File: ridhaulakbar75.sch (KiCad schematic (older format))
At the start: 204 parts, among them J1 Conn_01x04, J2 AVR-ISP-6, U1 TEENSY2.0

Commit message: big update
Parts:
- removed C1, C10, C11, C12, C13, C14, C15, C16, C17, C18, C2, C3, C4, C5, C6, C7, C8, C9: 0.1uF, Capacitor_SMD:C_0603_1608Metric_Pad1.05x0.95mm_HandSolder, symbol Device:C_Small
- removed D71: 1N4148W, master-Keebio-Parts:D_SOD-123-v2, symbol Diode:1N4148W
- removed J2: AVR-ISP-6, random-keyboard-parts:Reset_Pretty-Mask, symbol Connector:AVR-ISP-6
- removed LED1, LED10, LED11, LED12, LED13, LED14, LED15, LED16, LED17, LED18, LED2, LED3, LED4, LED5, LED6, LED7, LED8, LED9: WS2812B, WS2812B:WS2812B, symbol ws2812b:WS2812B
- removed MX71: Prnt Scr, MX_Only:MXOnly-1U-NoLED, symbol MX_Alps_Hybrid:MX-NoLED
- removed U1: TEENSY2.0, master-Keebio-Parts:Teensy_2.0, symbol keyboard_parts:TEENSY2.0
- added D82: BLUE, LED_SMD:LED_0603_1608Metric, symbol Device:LED
- added D83: 1N5819, Diode_SMD:D_SOD-323F, symbol Device:D_Schottky_Small
- added D84: RED, LED_SMD:LED_0603_1608Metric, symbol Device:LED
- added F1: 500mA, Fuse:Fuse_1206_3216Metric, symbol Device:Polyfuse_Small
- added J2: Ex_Bat, Connector_PinHeader_2.54mm:PinHeader_1x02_P2.54mm_Vertical, symbol Connector_Generic:Conn_01x02
- added J3: Ex_USB, nrfmicro:connector_usb, symbol Connector_Generic:Conn_01x04
- added Q1, Q2: AO3407, Package_TO_SOT_SMD:SOT-23, symbol Device:Q_PMOS_GSD
- added R1, R2: 5.1k, Resistor_SMD:R_0603_1608Metric, symbol Device:R_Small
- added R3: 820K, Resistor_SMD:R_0603_1608Metric, symbol Device:R_Small
- added R4, R8: 1K, Resistor_SMD:R_0603_1608Metric, symbol Device:R_Small
- added R5, R6: 2M, Resistor_SMD:R_0603_1608Metric, symbol Device:R_Small
- added R7: 100k, Resistor_SMD:R_0603_1608Metric, symbol Device:R_Small
- added R9: 2K, Resistor_SMD:R_0603_1608Metric, symbol Device:R_Small
- added SW1: Rotary_Encoder_Switch, master-Keebio-Parts:RotaryEncoder_EC11-no-legs, symbol Device:Rotary_Encoder_Switch
- added U1: USBLC6-2SC6, Package_TO_SOT_SMD:SOT-23-6, symbol Power_Protection:USBLC6-2SC6
- added U2: E73-2G4M08S1C-52840, nrfmicro:E73-2G4M08S1C-52840, symbol nrfmicro:E73-2G4M08S1C-52840
- added U3: XC6220B331MR, Package_TO_SOT_SMD:SOT-23-5, symbol Regulator_Linear:XC6220B331MR
- added U4: TP4054, Package_TO_SOT_SMD:SOT-23-5, symbol Battery_Management:MCP73831-3-OT
- added Y1: 32.768kHz, Crystal:Crystal_SMD_MicroCrystal_CM9V-T1A-2Pin_1.6x1.0mm, symbol Device:Crystal_Small
- J1: value Conn_01x04 -> SWD; footprint Connector_PinHeader_2.54mm:PinHeader_1x04_P2.54mm_Vertical -> nrfmicro:connector_swd
- MX1, MX18: footprint MX_Only:MXOnly-1U-NoLED -> MX_Only:MXOnly-1U-Hotswap
- MX10: renamed from MX49; footprint MX_Only:MXOnly-1U-NoLED -> MX_Only:MXOnly-1U-Hotswap
- MX11: renamed from MX54; footprint MX_Only:MXOnly-1U-NoLED -> MX_Only:MXOnly-1U-Hotswap
- MX12: renamed from MX60; footprint MX_Only:MXOnly-1U-NoLED -> MX_Only:MXOnly-1U-Hotswap
- MX13: renamed from MX66; footprint MX_Only:MXOnly-1U-NoLED -> MX_Only:MXOnly-1U-Hotswap
- MX14: renamed from MX77; footprint MX_Only:MXOnly-1U-NoLED -> MX_Only:MXOnly-1U-Hotswap
- MX15: renamed from MX2; footprint MX_Only:MXOnly-1U-NoLED -> MX_Only:MXOnly-1U-Hotswap
- MX16: renamed from MX8; footprint MX_Only:MXOnly-1U-NoLED -> MX_Only:MXOnly-1U-Hotswap
- MX17: renamed from MX13; footprint MX_Only:MXOnly-1U-NoLED -> MX_Only:MXOnly-1U-Hotswap
- MX19: renamed from MX24; footprint MX_Only:MXOnly-1U-NoLED -> MX_Only:MXOnly-1U-Hotswap
- MX2: renamed from MX7; footprint MX_Only:MXOnly-1U-NoLED -> MX_Only:MXOnly-1U-Hotswap
- MX20: renamed from MX29; footprint MX_Only:MXOnly-1U-NoLED -> MX_Only:MXOnly-1U-Hotswap
- MX21: renamed from MX34; footprint MX_Only:MXOnly-1U-NoLED -> MX_Only:MXOnly-1U-Hotswap
- MX22: renamed from MX40; footprint MX_Only:MXOnly-1U-NoLED -> MX_Only:MXOnly-1U-Hotswap
- MX23: renamed from MX45; footprint MX_Only:MXOnly-1U-NoLED -> MX_Only:MXOnly-1U-Hotswap
- MX24: renamed from MX50; footprint MX_Only:MXOnly-1U-NoLED -> MX_Only:MXOnly-1U-Hotswap
- MX25: renamed from MX55; footprint MX_Only:MXOnly-1U-NoLED -> MX_Only:MXOnly-1U-Hotswap
- MX26: renamed from MX61; footprint MX_Only:MXOnly-1U-NoLED -> MX_Only:MXOnly-1U-Hotswap
- MX27: renamed from MX67; footprint MX_Only:MXOnly-1U-NoLED -> MX_Only:MXOnly-1U-Hotswap
- MX28: renamed from MX72; footprint MX_Only:MXOnly-2U-NoLED -> MX_Only:MXOnly-2U-Hotswap
- MX29: renamed from MX78; footprint MX_Only:MXOnly-1U-NoLED -> MX_Only:MXOnly-1U-Hotswap
- MX3: renamed from MX12; footprint MX_Only:MXOnly-1U-NoLED -> MX_Only:MXOnly-1U-Hotswap
- MX30: renamed from MX3; footprint MX_Only:MXOnly-1.5U-NoLED -> MX_Only:MXOnly-1.5U-Hotswap
- MX31: renamed from MX9; footprint MX_Only:MXOnly-1U-NoLED -> MX_Only:MXOnly-1U-Hotswap
- MX32: renamed from MX14; footprint MX_Only:MXOnly-1U-NoLED -> MX_Only:MXOnly-1U-Hotswap
- MX33: renamed from MX19; footprint MX_Only:MXOnly-1U-NoLED -> MX_Only:MXOnly-1U-Hotswap
- MX34: renamed from MX25; footprint MX_Only:MXOnly-1U-NoLED -> MX_Only:MXOnly-1U-Hotswap
- MX35: renamed from MX30; footprint MX_Only:MXOnly-1U-NoLED -> MX_Only:MXOnly-1U-Hotswap
- MX36: renamed from MX35; footprint MX_Only:MXOnly-1U-NoLED -> MX_Only:MXOnly-1U-Hotswap
- MX37: renamed from MX41; footprint MX_Only:MXOnly-1U-NoLED -> MX_Only:MXOnly-1U-Hotswap
- MX38: renamed from MX46; footprint MX_Only:MXOnly-1U-NoLED -> MX_Only:MXOnly-1U-Hotswap
- MX39: renamed from MX51; footprint MX_Only:MXOnly-1U-NoLED -> MX_Only:MXOnly-1U-Hotswap
- MX4: renamed from MX17; footprint MX_Only:MXOnly-1U-NoLED -> MX_Only:MXOnly-1U-Hotswap
- MX40: renamed from MX56; footprint MX_Only:MXOnly-1U-NoLED -> MX_Only:MXOnly-1U-Hotswap
- MX41: renamed from MX62; footprint MX_Only:MXOnly-1U-NoLED -> MX_Only:MXOnly-1U-Hotswap
- MX42: renamed from MX68; footprint MX_Only:MXOnly-1U-NoLED -> MX_Only:MXOnly-1U-Hotswap
- MX43: renamed from MX73; footprint MX_Only:MXOnly-1.5U-NoLED -> MX_Only:MXOnly-1.5U-Hotswap
- MX44: renamed from MX79; footprint MX_Only:MXOnly-1U-NoLED -> MX_Only:MXOnly-1U-Hotswap
- MX45: renamed from MX4; footprint MX_Only:MXOnly-1.75U-NoLED -> MX_Only:MXOnly-1.75U-Hotswap
- MX46: renamed from MX10; footprint MX_Only:MXOnly-1U-NoLED -> MX_Only:MXOnly-1U-Hotswap
- MX47: renamed from MX15; footprint MX_Only:MXOnly-1U-NoLED -> MX_Only:MXOnly-1U-Hotswap
- MX48: renamed from MX20; footprint MX_Only:MXOnly-1U-NoLED -> MX_Only:MXOnly-1U-Hotswap
- MX49: renamed from MX26; footprint MX_Only:MXOnly-1U-NoLED -> MX_Only:MXOnly-1U-Hotswap
- MX5: renamed from MX23; footprint MX_Only:MXOnly-1U-NoLED -> MX_Only:MXOnly-1U-Hotswap
- MX50: renamed from MX31; footprint MX_Only:MXOnly-1U-NoLED -> MX_Only:MXOnly-1U-Hotswap
- MX51: renamed from MX36; footprint MX_Only:MXOnly-1U-NoLED -> MX_Only:MXOnly-1U-Hotswap
- MX52: renamed from MX42; footprint MX_Only:MXOnly-1U-NoLED -> MX_Only:MXOnly-1U-Hotswap
- MX53: renamed from MX47; footprint MX_Only:MXOnly-1U-NoLED -> MX_Only:MXOnly-1U-Hotswap
- MX54: renamed from MX52; footprint MX_Only:MXOnly-1U-NoLED -> MX_Only:MXOnly-1U-Hotswap
- MX55: renamed from MX57; footprint MX_Only:MXOnly-1U-NoLED -> MX_Only:MXOnly-1U-Hotswap
- MX56: renamed from MX63; footprint MX_Only:MXOnly-1U-NoLED -> MX_Only:MXOnly-1U-Hotswap
- MX57: renamed from MX74; footprint MX_Only:MXOnly-2.25U-NoLED -> MX_Only:MXOnly-2.25U-Hotswap
- MX58: renamed from MX80; footprint MX_Only:MXOnly-1U-NoLED -> MX_Only:MXOnly-1U-Hotswap
- MX59: renamed from MX5; footprint MX_Only:MXOnly-2.25U-NoLED -> MX_Only:MXOnly-2.25U-Hotswap
- MX6: renamed from MX28; footprint MX_Only:MXOnly-1U-NoLED -> MX_Only:MXOnly-1U-Hotswap
- MX60: renamed from MX16; footprint MX_Only:MXOnly-1U-NoLED -> MX_Only:MXOnly-1U-Hotswap
- MX61: renamed from MX21; footprint MX_Only:MXOnly-1U-NoLED -> MX_Only:MXOnly-1U-Hotswap
- MX62: renamed from MX27; footprint MX_Only:MXOnly-1U-NoLED -> MX_Only:MXOnly-1U-Hotswap
- MX63: renamed from MX32; footprint MX_Only:MXOnly-1U-NoLED -> MX_Only:MXOnly-1U-Hotswap
- MX64: renamed from MX37; footprint MX_Only:MXOnly-1U-NoLED -> MX_Only:MXOnly-1U-Hotswap
- MX65: renamed from MX43; footprint MX_Only:MXOnly-1U-NoLED -> MX_Only:MXOnly-1U-Hotswap
- MX66: renamed from MX48; footprint MX_Only:MXOnly-1U-NoLED -> MX_Only:MXOnly-1U-Hotswap
- MX67: renamed from MX53; footprint MX_Only:MXOnly-1U-NoLED -> MX_Only:MXOnly-1U-Hotswap
- MX68: renamed from MX58; footprint MX_Only:MXOnly-1U-NoLED -> MX_Only:MXOnly-1U-Hotswap
- MX69: renamed from MX64; footprint MX_Only:MXOnly-1U-NoLED -> MX_Only:MXOnly-1U-Hotswap
- MX7: renamed from MX33; footprint MX_Only:MXOnly-1U-NoLED -> MX_Only:MXOnly-1U-Hotswap
- MX70: renamed from MX69; footprint MX_Only:MXOnly-1.75U-NoLED -> MX_Only:MXOnly-1.75U-Hotswap
- MX71: renamed from MX75; footprint MX_Only:MXOnly-1U-NoLED -> MX_Only:MXOnly-1U-Hotswap
- MX72: renamed from MX81; footprint MX_Only:MXOnly-1U-NoLED -> MX_Only:MXOnly-1U-Hotswap
- MX73: renamed from MX6; footprint MX_Only:MXOnly-1.5U-NoLED -> MX_Only:MXOnly-1.25U-Hotswap
- MX74: renamed from MX11; footprint MX_Only:MXOnly-1U-NoLED -> MX_Only:MXOnly-1.25U-Hotswap
- MX75: renamed from MX22; footprint MX_Only:MXOnly-1.5U-NoLED -> MX_Only:MXOnly-1.25U-Hotswap
- MX76: renamed from MX38; footprint MX_Only:MXOnly-7U-NoLED -> MX_Only:MXOnly-6.25U-Hotswap-ReversedStabilizers
- MX77: renamed from MX59; footprint MX_Only:MXOnly-1U-NoLED -> MX_Only:MXOnly-1.25U-Hotswap
- MX78: renamed from MX65; footprint MX_Only:MXOnly-1U-NoLED -> MX_Only:MXOnly-1.25U-Hotswap
- MX79: renamed from MX70; footprint MX_Only:MXOnly-1U-NoLED -> MX_Only:MXOnly-1U-Hotswap
- MX8: renamed from MX39; footprint MX_Only:MXOnly-1U-NoLED -> MX_Only:MXOnly-1U-Hotswap
- MX80: renamed from MX76; footprint MX_Only:MXOnly-1U-NoLED -> MX_Only:MXOnly-1U-Hotswap
- MX81: renamed from MX82; footprint MX_Only:MXOnly-1U-NoLED -> MX_Only:MXOnly-1U-Hotswap
- MX9: renamed from MX44; footprint MX_Only:MXOnly-1U-NoLED -> MX_Only:MXOnly-1U-Hotswap
- USB1: footprint master-Keebio-Parts:HRO-TYPE-C-31-M-12-Assembly -> Type-C:HRO-TYPE-C-31-M-12-HandSoldering
- renumbered D49 to D10, D54 to D11, D60 to D12, D66 to D13, D77 to D14, D2 to D15, D8 to D16, D13 to D17, D24 to D19, D7 to D2, D29 to D20, D34 to D21, D40 to D22, D45 to D23, D50 to D24, D55 to D25, D61 to D26, D67 to D27, D72 to D28, D78 to D29, D12 to D3, D3 to D30, D9 to D31, D14 to D32, D19 to D33, D25 to D34, D30 to D35, D35 to D36, D41 to D37, D46 to D38, D51 to D39, D17 to D4, D56 to D40, D62 to D41, D68 to D42, D73 to D43, D79 to D44, D4 to D45, D10 to D46, D15 to D47, D20 to D48, D26 to D49, D23 to D5, D31 to D50, D36 to D51, D42 to D52, D47 to D53, D52 to D54, D57 to D55, D63 to D56, D74 to D57, D80 to D58, D5 to D59, D28 to D6, D16 to D60, D21 to D61, D27 to D62, D32 to D63, D37 to D64, D43 to D65, D48 to D66, D53 to D67, D58 to D68, D64 to D69, D33 to D7, D69 to D70, D75 to D71, D81 to D72, D6 to D73, D11 to D74, D22 to D75, D38 to D76, D59 to D77, D65 to D78, D70 to D79, D39 to D8, D76 to D80, D82 to D81, D44 to D9
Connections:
- net labels added: BATTERY_PIN, BLUE_LED, CC1, CC2, COL15, DATA+, DATA-, DCCH, EXT_VCC, POWER_PIN, PROG, RESET, Rotary-A, Rotary-B, SWC, SWD, VBAT, nRF_VDD
- net labels removed: +5V, D+, D-, DM-USB, DP-USB, GND-USB, MISO, MOSI, RGB, RST, SCK, VBUS-USB, VCC
- wire segments 506 -> 328
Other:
- note added: "LiPo Charging"
- note added: "Power & Filtering"
- moved on the sheet: D10, D11, D12, D13, D14, D6, D60, D61, D62, D63, D64, D65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

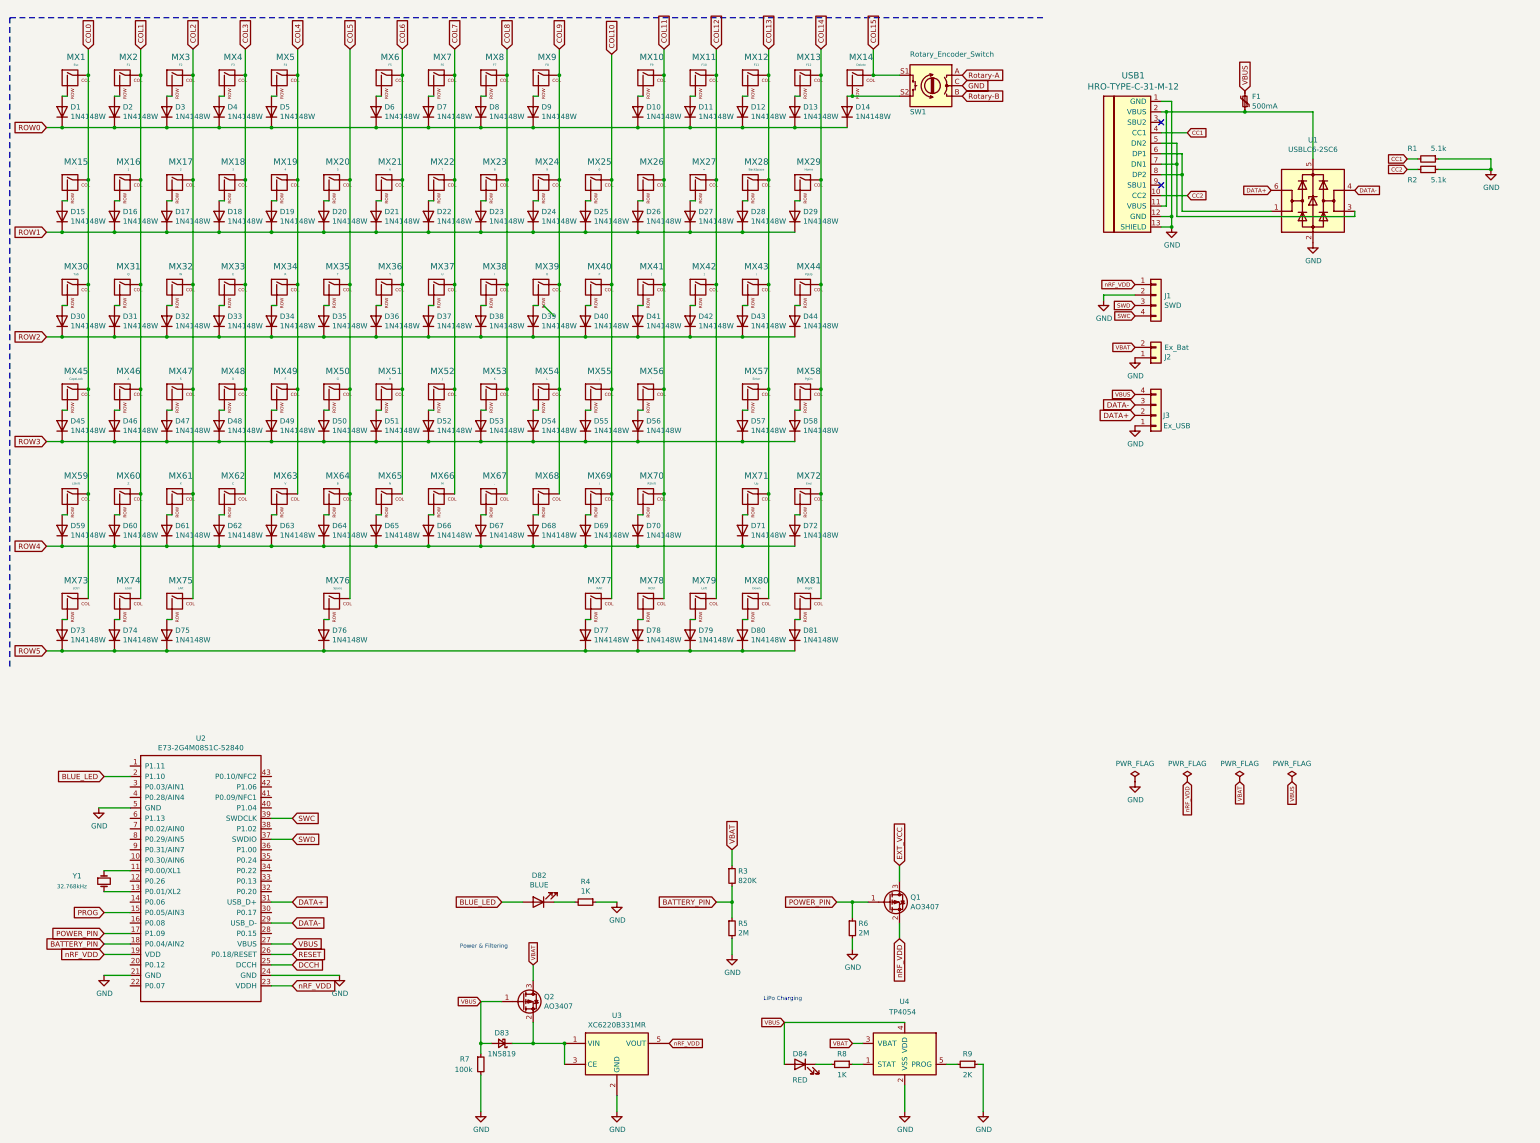
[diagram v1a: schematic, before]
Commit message: updae
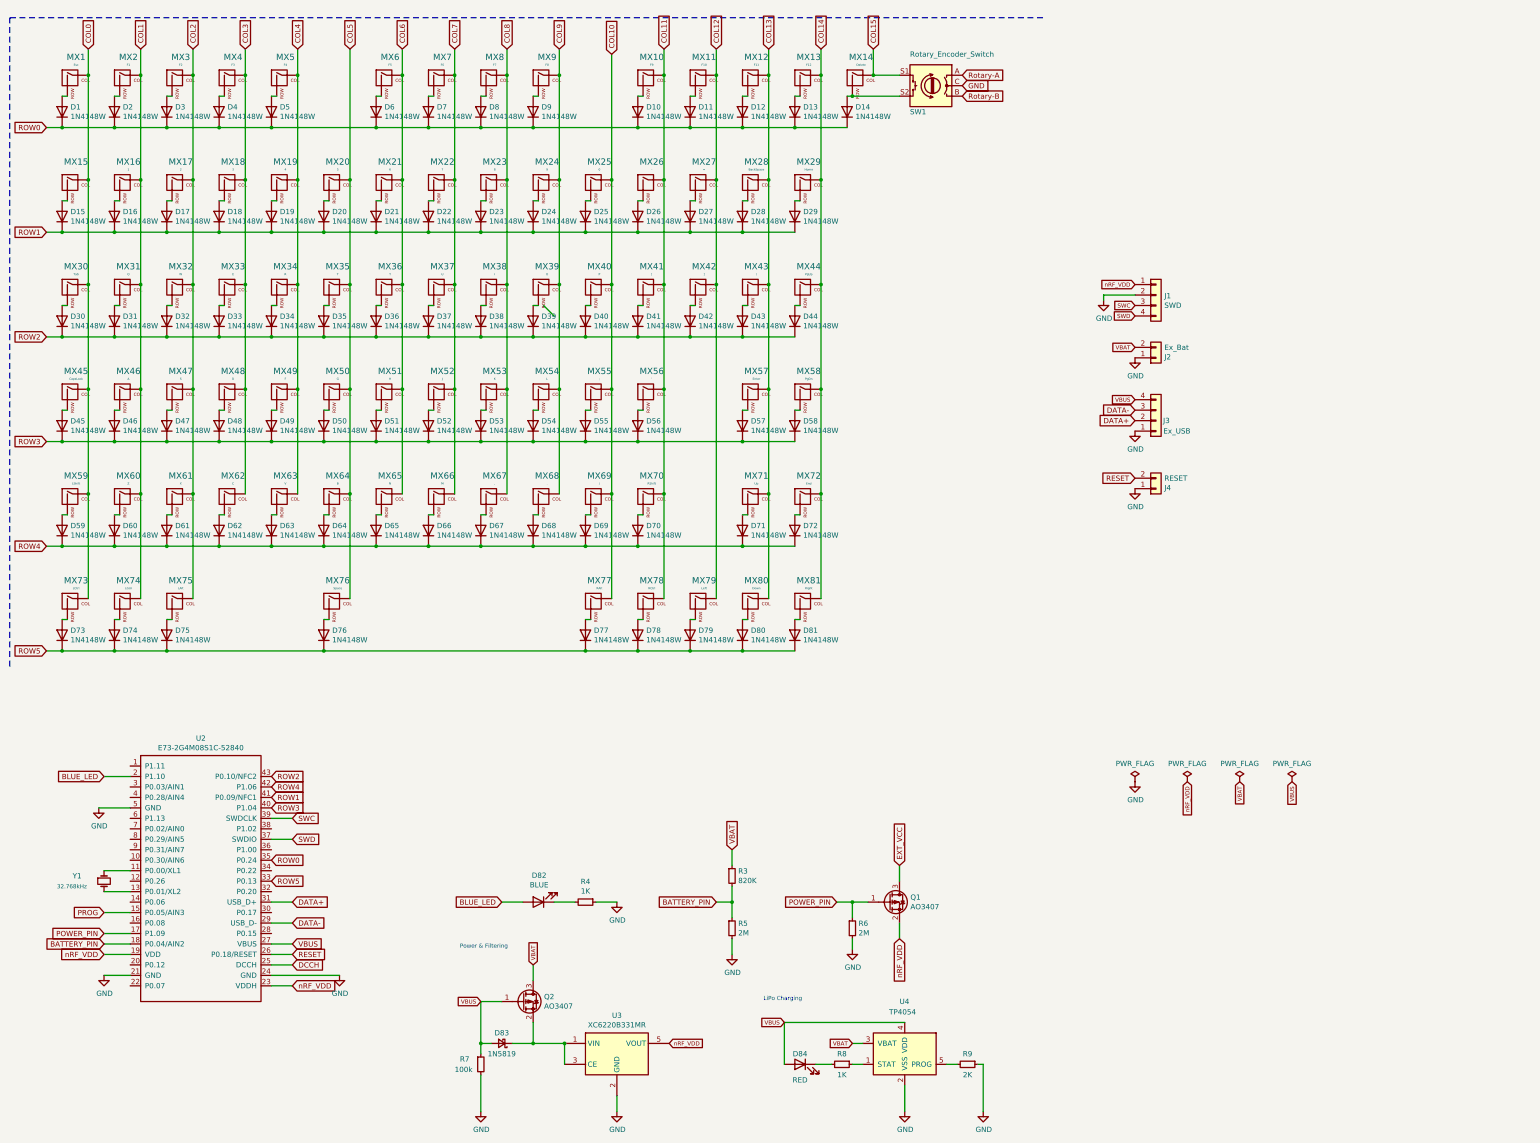
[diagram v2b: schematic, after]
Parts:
- removed F1: 500mA, Fuse:Fuse_1206_3216Metric, symbol Device:Polyfuse_Small
- removed R1, R2: 5.1k, Resistor_SMD:R_0603_1608Metric, symbol Device:R_Small
- removed U1: USBLC6-2SC6, Package_TO_SOT_SMD:SOT-23-6, symbol Power_Protection:USBLC6-2SC6
- removed USB1: HRO-TYPE-C-31-M-12, Type-C:HRO-TYPE-C-31-M-12-HandSoldering, symbol keebio:HRO-TYPE-C-31-M-12
- added J4: RESET, random-keyboard-parts:PushButton_6x6mm_TH, symbol Connector_Generic:Conn_01x02
- J2: footprint Connector_PinHeader_2.54mm:PinHeader_1x02_P2.54mm_Vertical -> Connector_JST:JST_SH_BM02B-SRSS-TB_1x02-1MP_P1.00mm_Vertical
- J3: footprint nrfmicro:connector_usb -> Connector_JST:JST_SH_BM04B-SRSS-TB_1x04-1MP_P1.00mm_Vertical
- MX1, MX10, MX11, MX12, MX13, MX14, MX15, MX16, MX17, MX18, MX19, MX2, MX20, MX21, MX22, MX23, MX24, MX25, MX26, MX27, MX29, MX3, MX31, MX32, MX33, MX34, MX35, MX36, MX37, MX38, MX39, MX4, MX40, MX41, MX42, MX44, MX46, MX47, MX48, MX49, MX5, MX50, MX51, MX52, MX53, MX54, MX55, MX56, MX58, MX6, MX60, MX61, MX62, MX63, MX64, MX65, MX66, MX67, MX68, MX69, MX7, MX71, MX72, MX79, MX8, MX80, MX81, MX9: footprint MX_Only:MXOnly-1U-Hotswap -> MX_Only:MXOnly-1U-NoLED
- MX28: footprint MX_Only:MXOnly-2U-Hotswap -> MX_Only:MXOnly-2U-NoLED
- MX30, MX43: footprint MX_Only:MXOnly-1.5U-Hotswap -> MX_Only:MXOnly-1.5U-NoLED
- MX45, MX70: footprint MX_Only:MXOnly-1.75U-Hotswap -> MX_Only:MXOnly-1.75U-NoLED
- MX57, MX59: footprint MX_Only:MXOnly-2.25U-Hotswap -> MX_Only:MXOnly-2.25U-NoLED
- MX73, MX74, MX75, MX77, MX78: footprint MX_Only:MXOnly-1.25U-Hotswap -> MX_Only:MXOnly-1.25U-NoLED
- MX76: footprint MX_Only:MXOnly-6.25U-Hotswap-ReversedStabilizers -> MX_Only:MXOnly-6.25U-ReversedStabilizers-NoLED
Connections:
- net GND: now also J4.1 (Pin_1)
- net RESET: now also J4.2 (Pin_2)
- net ROW0: now also U2.35 (P0.24)
- net ROW1: now also U2.41 (P0.09/NFC1)
- net ROW2: now also U2.43 (P0.10/NFC2)
- net ROW3: now also U2.40 (P1.04)
- net ROW4: now also U2.42 (P1.06)
- net ROW5: now also U2.33 (P0.13)
- net SWC: now also J1.3 (Pin_3); no longer J1.4 (Pin_4)
- net SWD: now also J1.4 (Pin_4); no longer J1.3 (Pin_3)
- no-connect marks 2 -> 0
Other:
- moved on the sheet: J3
